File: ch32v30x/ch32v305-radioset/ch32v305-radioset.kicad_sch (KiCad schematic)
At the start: 27 parts, among them J1 USB_C_Receptacle_USB2.0_14P, J2 PGM, U1 CH32V305GBU6, U2 CH570Q, U3 RCLAMP0502N, Y1 8MHz

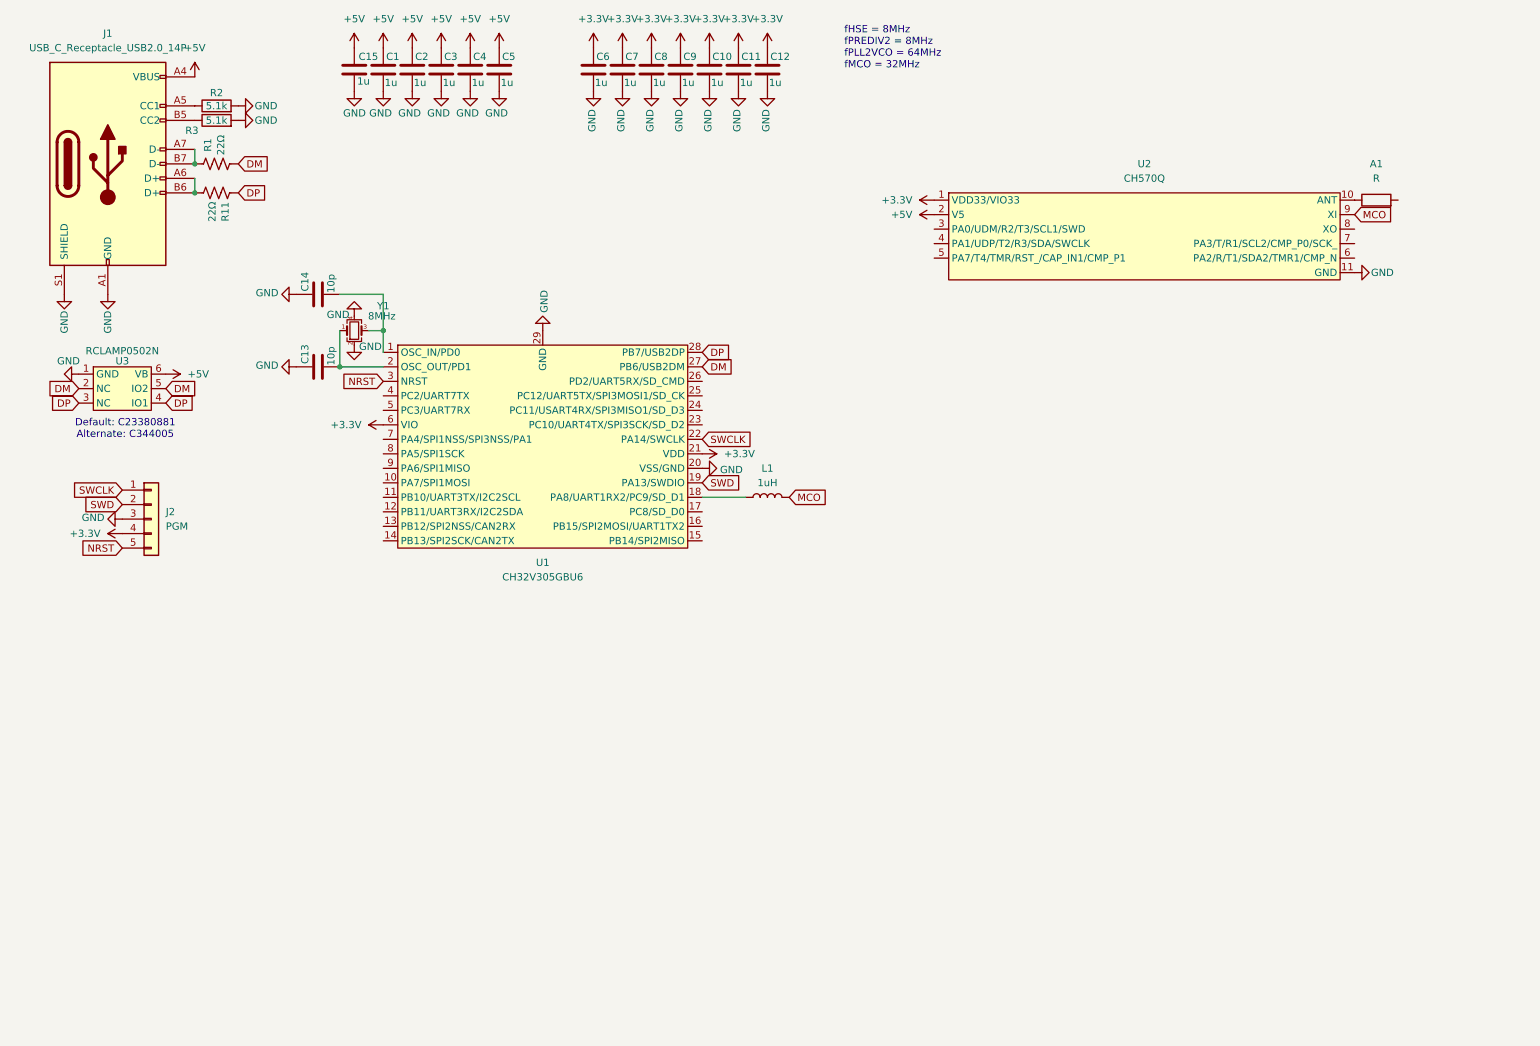
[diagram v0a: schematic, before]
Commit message: Bump all designs for order
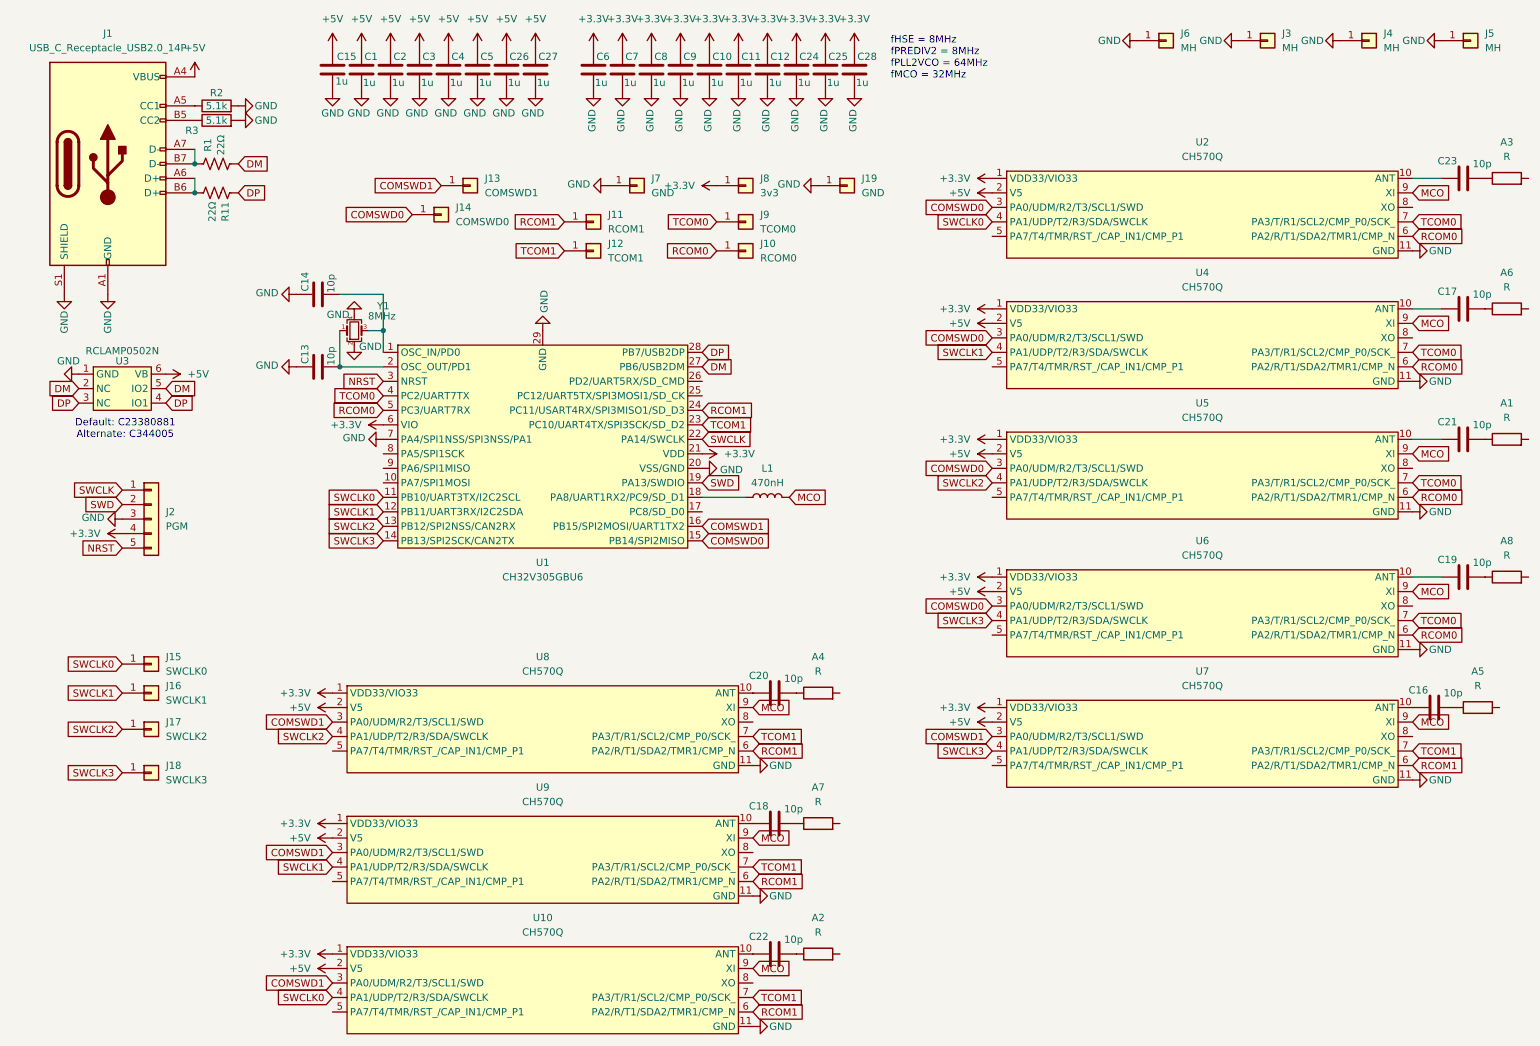
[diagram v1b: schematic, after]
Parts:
- added A2, A3, A4: R, RF_Antenna:Coilcraft_MA5532-AE_RFID, symbol Device:R
- added A5, A6, A7, A8: R, Resistor_SMD:R_2010_5025Metric, symbol Device:R
- added C16, C17, C18, C19, C20, C21, C22, C23: 10p, Capacitor_SMD:C_0402_1005Metric, symbol Device:C
- added C24, C25, C26, C27, C28: 1u, Capacitor_SMD:C_0402_1005Metric, symbol Device:C
- added J10: RCOM0, TestPoint:TestPoint_Pad_D1.5mm, symbol Connector_Generic:Conn_01x01
- added J11: RCOM1, TestPoint:TestPoint_Pad_D1.5mm, symbol Connector_Generic:Conn_01x01
- added J12: TCOM1, TestPoint:TestPoint_Pad_D1.5mm, symbol Connector_Generic:Conn_01x01
- added J13: COMSWD1, TestPoint:TestPoint_Pad_D1.5mm, symbol Connector_Generic:Conn_01x01
- added J14: COMSWD0, TestPoint:TestPoint_Pad_D1.5mm, symbol Connector_Generic:Conn_01x01
- added J15: SWCLK0, TestPoint:TestPoint_Pad_D1.5mm, symbol Connector_Generic:Conn_01x01
- added J16: SWCLK1, TestPoint:TestPoint_Pad_D1.5mm, symbol Connector_Generic:Conn_01x01
- added J17: SWCLK2, TestPoint:TestPoint_Pad_D1.5mm, symbol Connector_Generic:Conn_01x01
- added J18: SWCLK3, TestPoint:TestPoint_Pad_D1.5mm, symbol Connector_Generic:Conn_01x01
- added J19, J7: GND, TestPoint:TestPoint_Pad_D1.5mm, symbol Connector_Generic:Conn_01x01
- added J3, J4, J5, J6: MH, MountingHole:MountingHole_3.2mm_M3_DIN965_Pad, symbol Connector_Generic:Conn_01x01
- added J8: 3v3, TestPoint:TestPoint_Pad_D1.5mm, symbol Connector_Generic:Conn_01x01
- added J9: TCOM0, TestPoint:TestPoint_Pad_D1.5mm, symbol Connector_Generic:Conn_01x01
- added U10, U4, U5, U6, U7, U8, U9: CH570Q, Package_DFN_QFN:DFN-10-1EP_3x3mm_P0.5mm_EP1.7x2.5mm, symbol cnhardware:CH570Q
- A1: footprint Resistor_SMD:R_1206_3216Metric -> RF_Antenna:Coilcraft_MA5532-AE_RFID; LCSC C127629 -> C99665
- J1: footprint (none) -> cnhardware:USB_C_MOD_Receptacle_HRO_TYPE-C-31-M-12
- L1: value 1uH -> 470nH; LCSC C963789 -> C84476
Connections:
- net +3.3V: now also C24.1, C25.1, C28.1, J8.1 (Pin_1), U10.1 (VDD33/VIO33), U4.1 (VDD33/VIO33), U5.1 (VDD33/VIO33), U6.1 (VDD33/VIO33), U7.1 (VDD33/VIO33), U8.1 (VDD33/VIO33), U9.1 (VDD33/VIO33)
- net +5V: now also C26.1, C27.1, U10.2 (V5), U4.2 (V5), U5.2 (V5), U6.2 (V5), U7.2 (V5), U8.2 (V5), U9.2 (V5)
- net GND: now also U1.7 (PA4/SPI1NSS/SPI3NSS/PA1), C24.2, C25.2, C26.2, C27.2, C28.2, J19.1 (Pin_1), J3.1 (Pin_1), J4.1 (Pin_1), J5.1 (Pin_1), J6.1 (Pin_1), J7.1 (Pin_1), U10.11 (GND), U4.11 (GND), U5.11 (GND), U6.11 (GND), U7.11 (GND), U8.11 (GND), U9.11 (GND)
- net MCO: now also U10.9 (XI), U4.9 (XI), U5.9 (XI), U6.9 (XI), U7.9 (XI), U8.9 (XI), U9.9 (XI)
- net SWCLK0: now reaches U1.11 (PB10/UART3TX/I2C2SCL)
- net SWCLK0: now also U2.4 (PA1/UDP/T2/R3/SDA/SWCLK), J15.1 (Pin_1), U10.4 (PA1/UDP/T2/R3/SDA/SWCLK)
- net SWCLK1: now reaches U1.12 (PB11/UART3RX/I2C2SDA)
- net SWCLK1: now also J16.1 (Pin_1), U4.4 (PA1/UDP/T2/R3/SDA/SWCLK), U9.4 (PA1/UDP/T2/R3/SDA/SWCLK)
- net SWCLK2: now reaches U1.13 (PB12/SPI2NSS/CAN2RX)
- net SWCLK2: now also J17.1 (Pin_1), U5.4 (PA1/UDP/T2/R3/SDA/SWCLK), U8.4 (PA1/UDP/T2/R3/SDA/SWCLK)
- net SWCLK3: now reaches U1.14 (PB13/SPI2SCK/CAN2TX)
- net SWCLK3: now also J18.1 (Pin_1), U6.4 (PA1/UDP/T2/R3/SDA/SWCLK), U7.4 (PA1/UDP/T2/R3/SDA/SWCLK)
- net COMSWD0: now reaches U1.15 (PB14/SPI2MISO)
- net COMSWD0: now also U2.3 (PA0/UDM/R2/T3/SCL1/SWD), J14.1 (Pin_1), U4.3 (PA0/UDM/R2/T3/SCL1/SWD), U5.3 (PA0/UDM/R2/T3/SCL1/SWD), U6.3 (PA0/UDM/R2/T3/SCL1/SWD)
- net COMSWD1: now reaches U1.16 (PB15/SPI2MOSI/UART1TX2)
- net COMSWD1: now also J13.1 (Pin_1), U10.3 (PA0/UDM/R2/T3/SCL1/SWD), U7.3 (PA0/UDM/R2/T3/SCL1/SWD), U8.3 (PA0/UDM/R2/T3/SCL1/SWD), U9.3 (PA0/UDM/R2/T3/SCL1/SWD)
- net TCOM1: now reaches U1.23 (PC10/UART4TX/SPI3SCK/SD_D2)
- net TCOM1: now also J12.1 (Pin_1), U10.7 (PA3/T/R1/SCL2/CMP_P0/SCK_), U7.7 (PA3/T/R1/SCL2/CMP_P0/SCK_), U8.7 (PA3/T/R1/SCL2/CMP_P0/SCK_), U9.7 (PA3/T/R1/SCL2/CMP_P0/SCK_)
- net RCOM1: now reaches U1.24 (PC11/USART4RX/SPI3MISO1/SD_D3)
- net RCOM1: now also J11.1 (Pin_1), U10.6 (PA2/R/T1/SDA2/TMR1/CMP_N), U7.6 (PA2/R/T1/SDA2/TMR1/CMP_N), U8.6 (PA2/R/T1/SDA2/TMR1/CMP_N), U9.6 (PA2/R/T1/SDA2/TMR1/CMP_N)
- net TCOM0: now reaches U1.4 (PC2/UART7TX)
- net TCOM0: now also U2.7 (PA3/T/R1/SCL2/CMP_P0/SCK_), J9.1 (Pin_1), U4.7 (PA3/T/R1/SCL2/CMP_P0/SCK_), U5.7 (PA3/T/R1/SCL2/CMP_P0/SCK_), U6.7 (PA3/T/R1/SCL2/CMP_P0/SCK_)
- net RCOM0: now reaches U1.5 (PC3/UART7RX)
- net RCOM0: now also U2.6 (PA2/R/T1/SDA2/TMR1/CMP_N), J10.1 (Pin_1), U4.6 (PA2/R/T1/SDA2/TMR1/CMP_N), U5.6 (PA2/R/T1/SDA2/TMR1/CMP_N), U6.6 (PA2/R/T1/SDA2/TMR1/CMP_N)
- net at A1.1: now also C21.2; no longer U2.10 (ANT)
- new net: C22.1, U10.10 (ANT)
- new net: A2.1, C22.2
- new net: C19.1, U6.10 (ANT)
- new net: C21.1, U5.10 (ANT)
- new net: C20.1, U8.10 (ANT)
- new net: C18.1, U9.10 (ANT)
- new net: A8.1, C19.2
- new net: C16.1, U7.10 (ANT)
- new net: A5.1, C16.2
- new net: A4.1, C20.2
- new net: A7.1, C18.2
- new net: C17.1, U4.10 (ANT)
- new net: A3.1, C23.2
- new net: C23.1, U2.10 (ANT)
- new net: A6.1, C17.2
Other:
- moved on the sheet: C1, C15, C2, C3, C4, C5, U2

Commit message: Bump design
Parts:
- U3: LCSC C23380881 -> C344005
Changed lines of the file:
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@@
 			)
 		)
-		(property "LCSC" "C23380881"
+		(property "LCSC" "C344005"
 			(at 33.02 80.01 0)
 			(effects
